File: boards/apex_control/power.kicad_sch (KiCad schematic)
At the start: 0 parts

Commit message: Logan done fo now
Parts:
- added C1, C2, C3, C4: C, symbol APEX_Symbols:C
- added L1: L, symbol APEX_Symbols:L
- added U6: MIMXRT1171DVMAB, APEX_FOOTPRINTS:MIMXRT1171DVMAB_BGA, symbol APEX_Symbols:MIMXRT1171DVMAB
- added U7: TPS62086, APEX_FOOTPRINTS:TPS62086_RLT0007A_TI, symbol APEX_Symbols:TPS62086
- added U8: TPS62825, APEX_FOOTPRINTS:TPS62825_DMQ0006A_TI, symbol APEX_Symbols:TPS62825
- added U9: LM66200, APEX_FOOTPRINTS:LM66200_DRL0008A_TI, symbol APEX_Symbols:LM66200
- added Y1: Crystal_GND24, APEX_FOOTPRINTS:XTAL_3225, symbol APEX_Symbols:Crystal_GND24
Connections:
- new net: L1.1, U7.6 (SW)
- new net: C4.1, U6.U16 (XTALI), Y1.4 (GND)
- new net: C3.1, U6.T16 (XTALO), Y1.2 (GND)
- new net: U6.A1 (VSS), U6.A17 (VSS), U6.B7 (VSS), U6.C10 (VSS), U6.C12 (VSS), U6.C14 (VSS), U6.C8 (VSS), U6.D4 (VSS), U6.F11 (VSS), U6.F12 (VSS), U6.F13 (VSS), U6.G10 (VSS), U6.G11 (VSS), U6.G15 (VSS), U6.G3 (VSS), U6.G7 (VSS), U6.G8 (VSS), U6.G9 (VSS), U6.H11 (VSS), U6.H7 (VSS), U6.J11 (VSS), U6.J7 (VSS), U6.K11 (VSS), U6.L10 (VSS), U6.L11 (VSS), U6.L15 (VSS), U6.L3 (VSS), U6.P14 (VSS), U6.P4 (VSS), U6.R4 (VSS), U6.R7 (VSS), U6.T12 (VSS), U6.U1 (VSS), U6.U17 (VSS)
- new net: U6.H10 (VDD_SOC_IN), U6.H8 (VDD_SOC_IN), U6.H9 (VDD_SOC_IN), U6.J10 (VDD_SOC_IN), U6.J8 (VDD_SOC_IN), U6.J9 (VDD_SOC_IN), U6.K10 (VDD_SOC_IN)
- new net: U6.K6 (DCDC_GND), U6.K7 (DCDC_GND), U6.L6 (DCDC_GND)
- new net: U6.K8 (DCDC_DIG), U6.K9 (DCDC_DIG), U6.L8 (DCDC_DIG)
- new net: U6.M5 (DCDC_IN), U6.N5 (DCDC_IN)
- new net: U6.M7 (DCDC_ANA), U6.M8 (DCDC_ANA)
- new net: U6.T3 (DCDC_LP), U6.U3 (DCDC_LP)
- new net: U6.T4 (DCDC_LN), U6.U4 (DCDC_LN)
- new net +1V8: U6.D12 (NVCC_DISP1), U6.D14 (NVCC_SD1), U6.E7 (NVCC_DISP2), U6.F6 (NVCC_EMC1), U6.F7 (NVCC_EMC1), U6.G13 (NVCC_SD2), U6.G16 (ADC_VREFH), U6.G6 (NVCC_EMC1), U6.P7 (NVCC_LPSR)
- new net +3V3_1: C2.2, L1.2, U6.G12 (VDD_USB_3P3), U6.H6 (NVCC_EMC2), U6.J13 (VDDA_ADC_3P3), U6.J6 (NVCC_EMC2), U6.M12 (NVCC_GPIO), U6.R12 (VDD_LPSR_IN), U7.3 (FB), U7.4 (VOS)
- new net +5V: C1.2, U7.1 (EN), U7.7 (VIN)
- new net GND: C1.1, C2.1, C3.2, C4.2, U7.5 (GND), Y1.1, Y1.3
- no-connect marks 0 -> 1

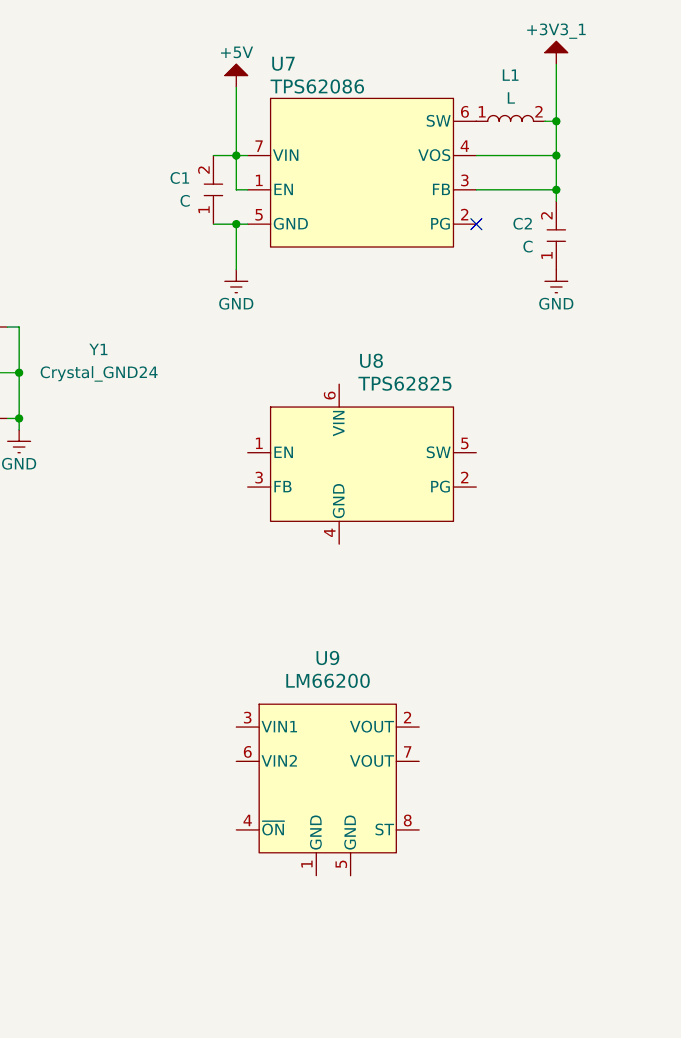
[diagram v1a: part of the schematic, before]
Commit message: More placement
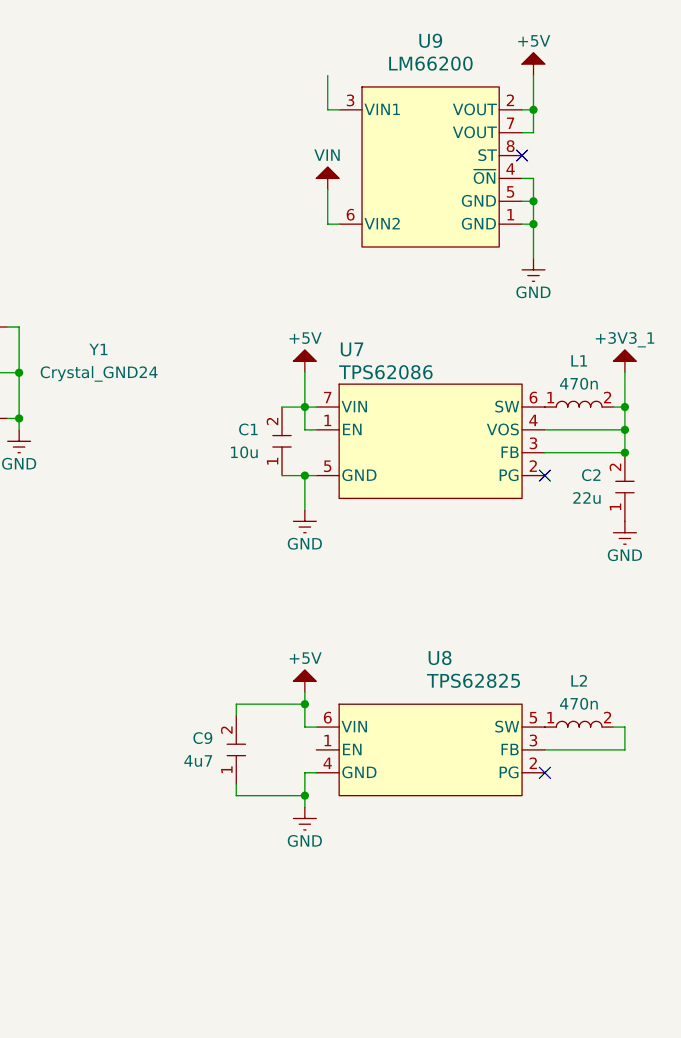
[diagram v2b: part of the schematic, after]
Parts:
- added C9: 4u7, symbol APEX_Symbols:C
- added L2: 470n, symbol APEX_Symbols:L
- C1: value C -> 10u
- C2: value C -> 22u
- L1: value L -> 470n
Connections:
- net +5V: now also U8.6 (VIN), U9.2 (VOUT), U9.7 (VOUT), C9.2
- net GND: now also U8.4 (GND), U9.1 (GND), U9.4 (~{ON}), U9.5 (GND), C9.1
- net at U8.3 (FB): now also L2.2
- net at U8.5 (SW): now also L2.1
- net VIN: now reaches U9.6 (VIN2)
- no-connect marks 1 -> 3
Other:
- moved on the sheet: C1, C2, L1, U7, U8, U9
